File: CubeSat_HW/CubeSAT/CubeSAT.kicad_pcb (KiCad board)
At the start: 2 copper layers, 85 x 56 mm, 17 parts, among them J1 Conn_01x10_Pin, J2 Conn_02x04_Odd_Even, J4 Conn_02x20_Odd_Even

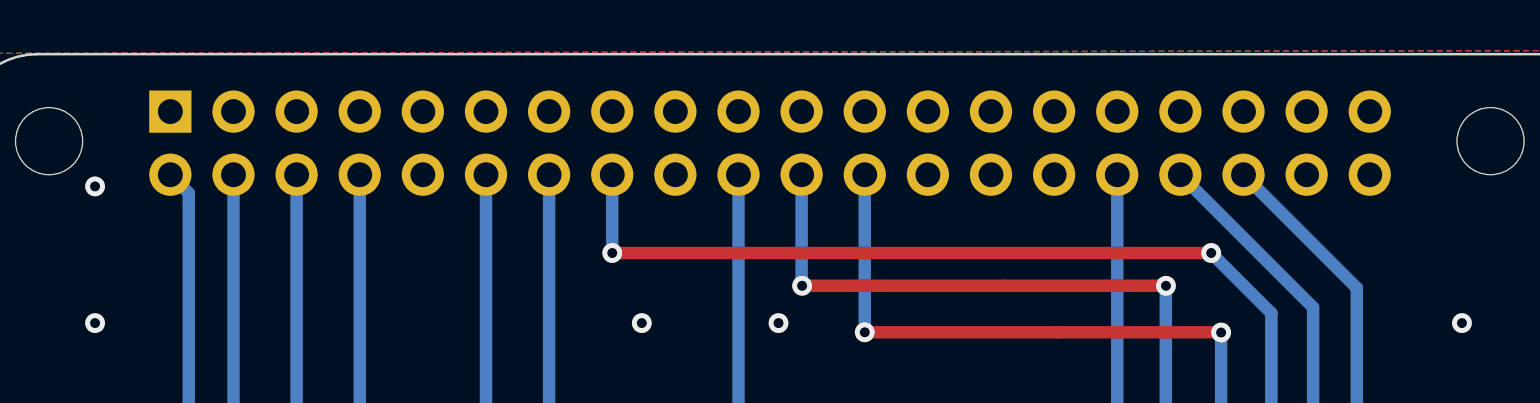
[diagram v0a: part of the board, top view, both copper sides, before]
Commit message: feat: Added new version for HW Board
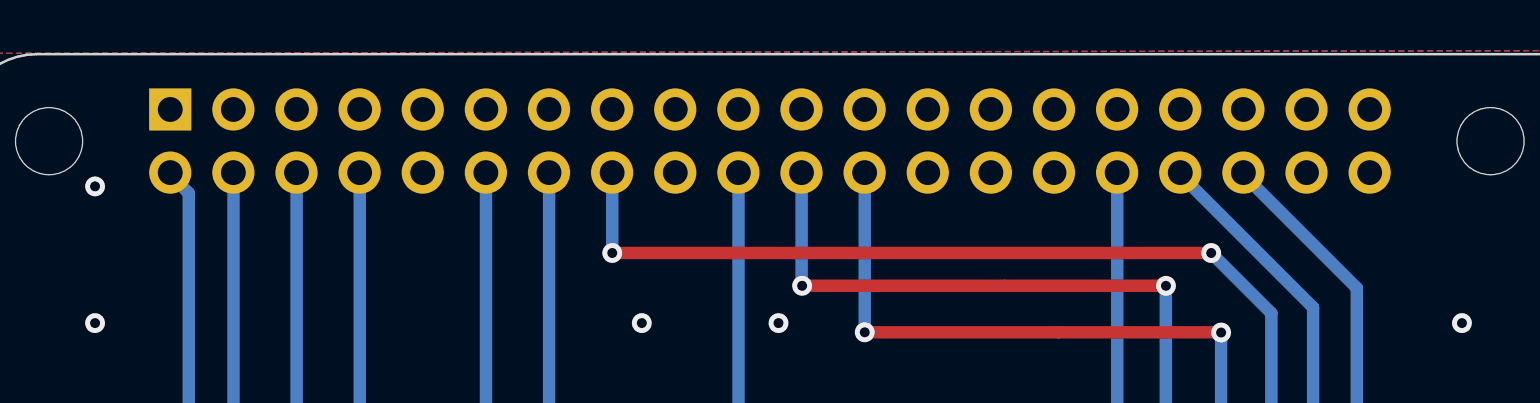
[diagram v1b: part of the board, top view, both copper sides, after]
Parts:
- moved J4 0.09 mm to (188.4, 62.2)
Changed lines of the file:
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@@
   )
   (footprint "Connector_PinHeader_2.54mm:PinHeader_2x20_P2.54mm_Vertical" (layer "B.Cu")
-    (at 188.38 62.31 -90)
+    (at 188.375 62.225 -90)
     (descr "Through hole straight pin header, 2x20, 2.54mm pitch, double rows")
     (tags "Through hole pin header THT 2x20 2.54mm double row")
